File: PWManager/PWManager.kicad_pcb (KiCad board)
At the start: 2 copper layers, 100 x 100 mm, 47 parts, among them J1 Conn_01x05, J2 USB_B_Micro, J3 UE27AC54100, SW1 SW_Push, SW2 SW_Push, SW3 SW_Push, U1 ATSAME51G18A-MFT, U2 BM71BLES1FC2-0B04AA, U3 M95640, U4 AP2138N-3.3TRG1

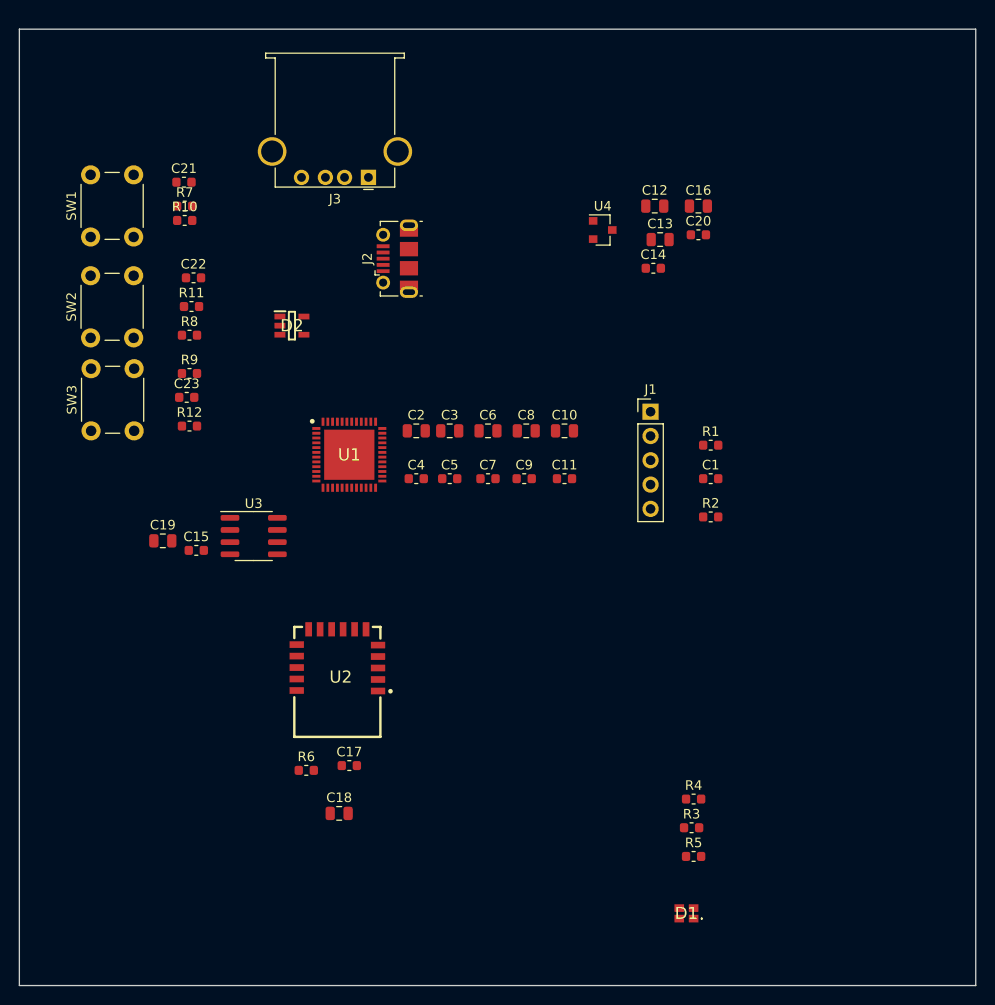
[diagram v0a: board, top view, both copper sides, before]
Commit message: Rev A Board
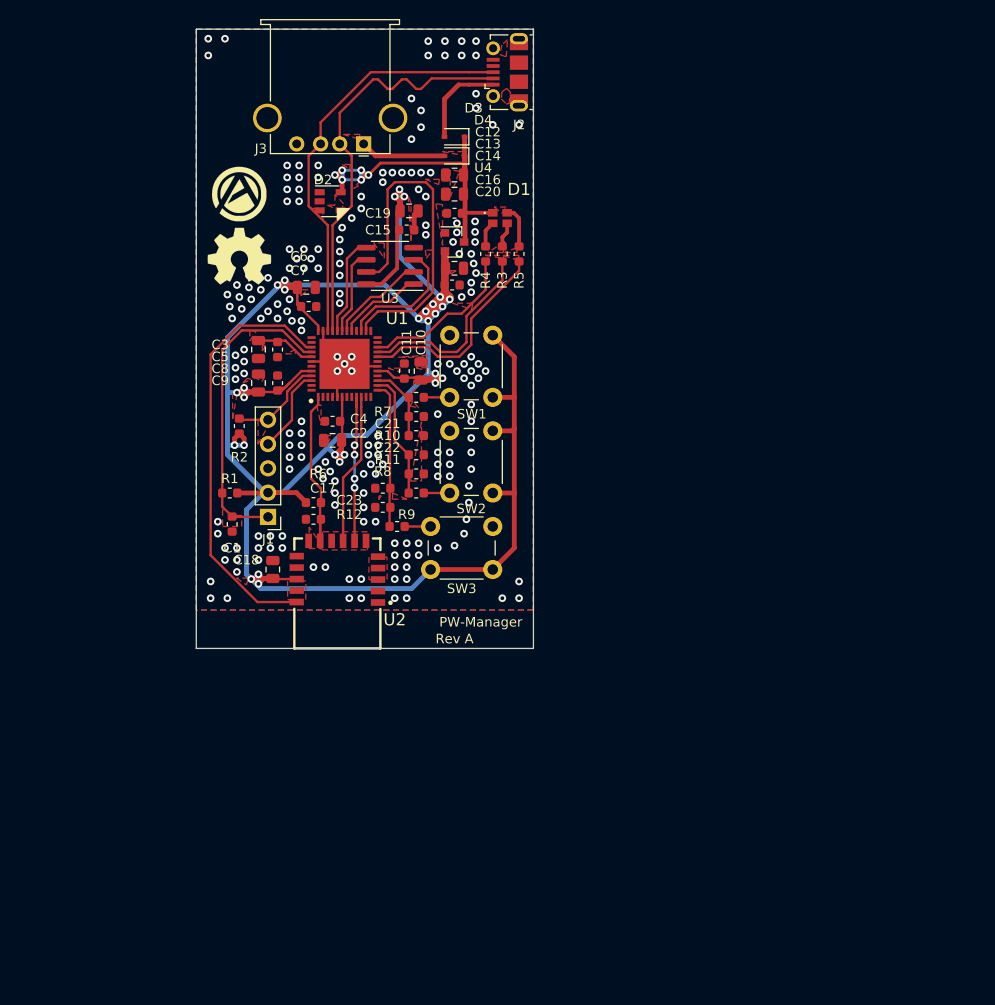
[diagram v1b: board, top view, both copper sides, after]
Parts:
- added D3: CUS08F30, Diode_SMD:D_SOD-323, F.Cu at (149.5, 33.2)
- added D4: CUS08F30, Diode_SMD:D_SOD-323, F.Cu at (149.5, 35.2)
- added G***: LOGO, silkprints:logo, F.Cu at (127.0, 39.2)
- added REF**: OSHW-Symbol_6.7x6mm_SilkScreen, Symbol:OSHW-Symbol_6.7x6mm_SilkScreen, F.Cu at (127.0, 45.8)
- D2: footprint SamacSys_Parts:SOT95P280X145-5N -> Package_TO_SOT_SMD:SOT-23-5
- moved D1 75.3 mm to (154.2, 41.8), turned to 180 degrees
- moved R5 65.6 mm to (156.2, 45.5), turned to 270 degrees
- moved R3 63.2 mm to (154.5, 45.5), turned to 270 degrees
- moved R4 61.0 mm to (152.8, 45.5), turned to 270 degrees
- moved R1 50.5 mm to (126.0, 70.5), turned to 180 degrees
- moved C1 50.3 mm to (126.2, 73.8), turned to 90 degrees
- moved R2 50.2 mm to (127.0, 63.5), turned to 270 degrees
- moved SW3 44.4 mm to (153.5, 78.5), turned to 180 degrees
- moved SW1 43.3 mm to (153.5, 54.0), turned to 270 degrees
- moved SW2 43.2 mm to (153.5, 64.0), turned to 270 degrees
- moved C19 43.1 mm to (144.8, 41.0)
- moved J1 41.5 mm to (130.0, 73.0), turned to 180 degrees
- moved C15 40.1 mm to (144.5, 43.0)
- moved C21 34.5 mm to (145.5, 62.5), turned to 180 degrees
- moved R10 33.1 mm to (145.5, 64.5), turned to 180 degrees
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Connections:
- C17 pad 1: RST -> RSTB
- J2 pad 1: +5V -> Net-(D3-Pad2)
- J3 pad 1: +5V -> Net-(D4-Pad2)
- R6 pad 2: RST -> RSTB
- U1 pad 1: Net-(U1-Pad1) -> RSTB
- U1 pad 10: Net-(U1-Pad10) -> TXD
- U1 pad 13: Net-(U1-Pad13) -> S2
- U1 pad 14: Net-(U1-Pad14) -> S1
- U1 pad 15: Net-(U1-Pad15) -> S0
- U1 pad 20: Net-(U1-Pad20) -> B
- U1 pad 21: Net-(U1-Pad21) -> G
- U1 pad 22: Net-(U1-Pad22) -> R
- U1 pad 26: Net-(U1-Pad26) -> Hold
- U1 pad 27: Net-(U1-Pad27) -> W
- U1 pad 29: Net-(U1-Pad29) -> S
- U1 pad 30: Net-(U1-Pad30) -> Q
- U1 pad 31: Net-(U1-Pad31) -> C
- U1 pad 32: Net-(U1-Pad32) -> D
- U1 pad 39: Net-(U1-Pad39) -> P2_0
- U1 pad 9: Net-(U1-Pad9) -> RXD
- U2 pad 10: RST -> RSTB
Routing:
- net VDD: track 0.00 -> 278.1 mm, vias 0 -> 28
- net P2_0: track 0.00 -> 44.8 mm
- net DP: track 0.00 -> 43.4 mm
- net DM: track 0.00 -> 43.3 mm
- net +5V: track 0.00 -> 40.5 mm, vias 0 -> 6
- net Hold: track 0.00 -> 35.6 mm
- net RST: track 0.00 -> 32.7 mm
- net B: track 0.00 -> 21.9 mm
- net G: track 0.00 -> 20.6 mm
- net RSTB: track 0.00 -> 18.2 mm
- net RXD: track 0.00 -> 17.2 mm, vias 0 -> 4
- net R: track 0.00 -> 16.7 mm
- net TXD: track 0.00 -> 15.8 mm
- net S2: track 0.00 -> 15.3 mm
- net W: track 0.00 -> 13.5 mm
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- added copper zone on F.Cu, net DM
- added copper zone on F.Cu, net DP
- added copper zone on B.Cu, net GND
- added copper zone on F.Cu, net GND
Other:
- board size 100 x 100 mm -> 35.2 x 64.8 mm
- board text added: "PW-Manager"
- board text added: "Rev A"
